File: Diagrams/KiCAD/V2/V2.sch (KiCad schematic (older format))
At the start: 10 parts

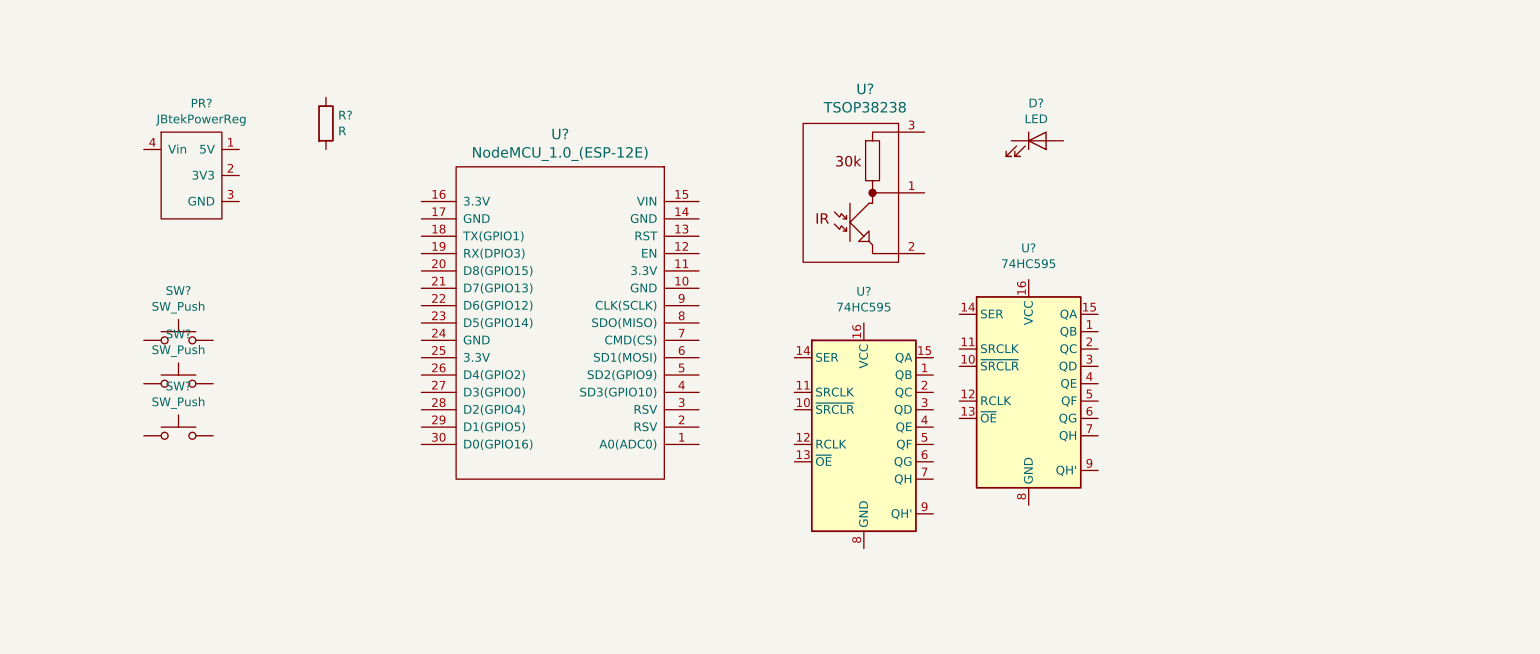
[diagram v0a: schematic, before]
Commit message: More work on KiCAD schematic. Believe it to be finished at this point.
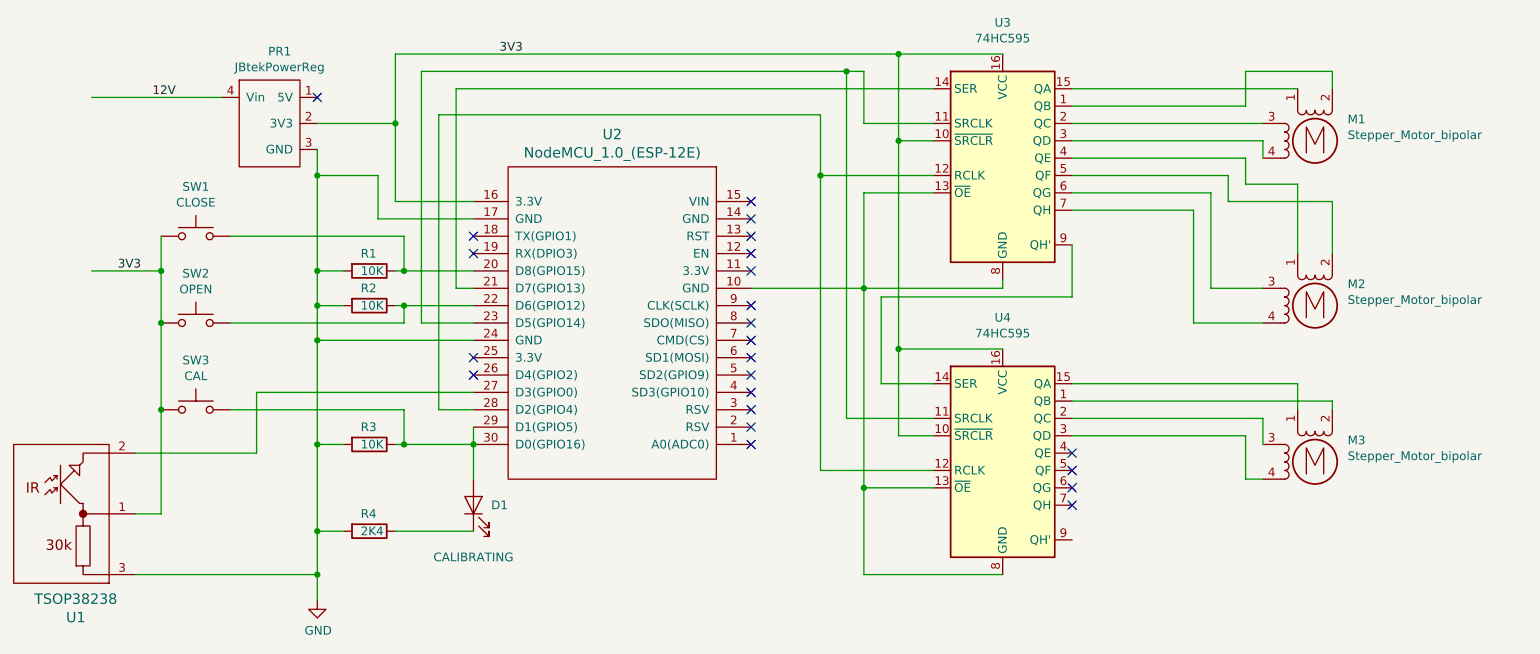
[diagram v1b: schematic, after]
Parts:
- removed PR?: JBtekPowerReg, symbol Kip_Custom_Lib:JBtekPowerReg
- added M1, M2, M3: Stepper_Motor_bipolar, symbol Motor:Stepper_Motor_bipolar
- added PR1: JBtekPowerReg, symbol Kip_Custom_Lib:JBtekPowerReg
- added R2, R3: 10K, symbol Device:R
- added R4: 2K4, symbol Device:R
- D1: renamed from D?; value LED -> CALIBRATING
- R1: renamed from R?; value R -> 10K
- SW1: renamed from SW?; value SW_Push -> CLOSE
- SW2: renamed from SW?; value SW_Push -> OPEN
- SW3: renamed from SW?; value SW_Push -> CAL
- gave numbers to parts that had none: 4
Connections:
- net at U2.10 (GND): now also U3.13 (~OE), U3.8 (GND), U4.13 (~OE), U4.8 (GND)
- net 3V3: now reaches U2.16 (3.3V)
- net 3V3: now also SW1.1, SW2.1, SW3.1, U1.1, U3.10 (~SRCLR), U3.16 (VCC), U4.10 (~SRCLR), U4.16 (VCC), PR1.2 (3V3)
- net GND: now reaches U2.17 (GND)
- net GND: now also R1.2, U1.3, U2.24 (GND), PR1.3 (GND), R2.2, R3.2, R4.2
- net at U2.20 (D8(GPIO15)): now also R1.1, SW1.2
- net at U2.21 (D7(GPIO13)): now also U3.14 (SER)
- net at U2.22 (D6(GPIO12)): now also SW2.2, R2.1
- net at U2.23 (D5(GPIO14)): now also U3.11 (SRCLK), U4.11 (SRCLK)
- net at U2.27 (D3(GPIO0)): now also U1.2
- net at U2.28 (D2(GPIO4)): now also U3.12 (RCLK), U4.12 (RCLK)
- net at U2.29 (D1(GPIO5)): now also D1.2 (A), SW3.2, U2.30 (D0(GPIO16)), R3.1
- net at U4.1 (QB): now also M3.2 (-)
- net at U4.14 (SER): now also U3.9 (QH')
- net at U4.15 (QA): now also M3.1
- net at U4.2 (QC): now also M3.3
- net at U4.3 (QD): now also M3.4
- net at U3.1 (QB): now also M1.2 (-)
- net at U3.15 (QA): now also M1.1
- net at U3.2 (QC): now also M1.3
- net at U3.3 (QD): now also M1.4
- net at U3.4 (QE): now also M2.1
- net at U3.5 (QF): now also M2.2 (-)
- net at U3.6 (QG): now also M2.3
- net at U3.7 (QH): now also M2.4
- net at D1.1 (K): now also R4.1
- new net 12V: PR1.4 (Vin)
- no-connect marks 0 -> 23
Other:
- moved on the sheet: D1, R1, SW1, SW2, SW3, U1, U2, U3, U4
